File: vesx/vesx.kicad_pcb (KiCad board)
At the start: 4 copper layers, 100 x 40 mm, 180 parts, among them J1 TYPE-C-31-M-12, J2 Conn_01x05, J3 Conn_01x06, J4 Conn_01x03, J5 Conn_01x04, J6 STLINK, J7 Conn_01x04, J8 CAN, U1 Opamp_Quad, U2 LM1117DT-3.3, U3 LM5164DDA, U4 TO220_replacement_module, U5 L6498DTR, U6 L6498DTR, U7 STM32F405RGTx, U8 L6498DTR, U9 SN65HVD230DR, Y2 8MHz

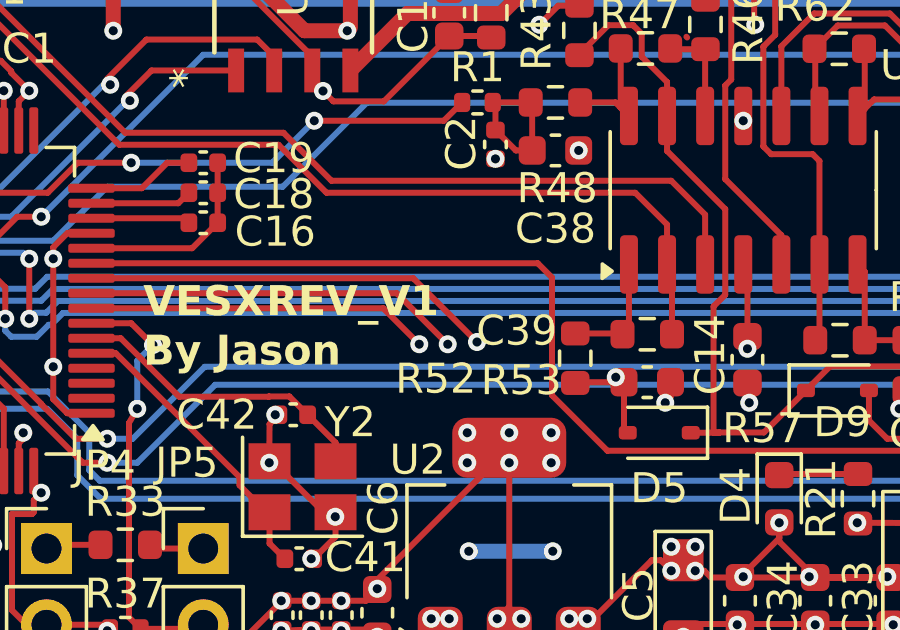
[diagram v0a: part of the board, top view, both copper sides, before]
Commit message: eeeeeeeeeeeeeeeeeeee
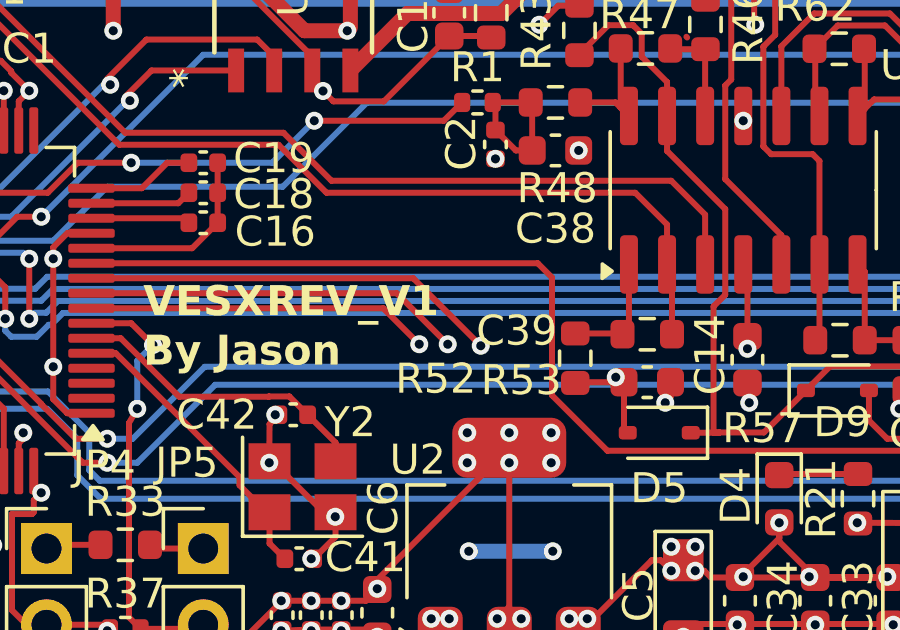
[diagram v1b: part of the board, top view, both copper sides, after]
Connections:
- C39 pad 1: CURRENT_A -> CURRENT_B
- C40 pad 1: CURRENT_B -> CURRENT_C
- D5 pad 2: CURRENT_A -> CURRENT_C
- R52 pad 2: CURRENT_A -> CURRENT_B
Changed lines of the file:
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@@
 			(layers "F.Cu" "F.Paste" "F.Mask")
 			(roundrect_rratio 0.25)
-			(net 48 "CURRENT_B")
+			(net 41 "CURRENT_C")
 			(pintype "passive")
 		)
@@
 			(layers "F.Cu" "F.Paste" "F.Mask")
 			(roundrect_rratio 0.25)
-			(net 34 "CURRENT_A")
+			(net 41 "CURRENT_C")
 			(pinfunction "A")
 			(pintype "passive")
@@
 			(layers "F.Cu" "F.Paste" "F.Mask")
 			(roundrect_rratio 0.25)
-			(net 34 "CURRENT_A")
+			(net 48 "CURRENT_B")
 			(pintype "passive")
 		)
@@
 			(layers "F.Cu" "F.Paste" "F.Mask")
 			(roundrect_rratio 0.25)
-			(net 34 "CURRENT_A")
+			(net 48 "CURRENT_B")
 			(pintype "passive")
 		)
@@
 	)
 	(segment
-		(start 197.925 41.775)
-		(end 195.8 39.65)
+		(start 195.8 39.65)
+		(end 185.075 39.65)
 		(width 0.2)
 		(layer "F.Cu")
@@
 	)
 	(segment
-		(start 213.2 36.34)
-		(end 212.8 36.74)
+		(start 198.05 41.9)
+		(end 195.8 39.65)
 		(width 0.2)
 		(layer "F.Cu")
@@
 	)
 	(segment
-		(start 195.8 39.65)
-		(end 185.075 39.65)
+		(start 213.2 36.34)
+		(end 212.8 36.74)
 		(width 0.2)
 		(layer "F.Cu")
@@
 	)
 	(via
-		(at 197.925 41.775)
+		(at 198.05 41.9)
 		(size 0.6)
 		(drill 0.3)
@@
 	)
 	(segment
-		(start 197.925 41.775)
-		(end 202.7 37)
+		(start 198.05 41.9)
+		(end 202.95 37)
 		(width 0.2)
 		(layer "In2.Cu")
@@
 	)
 	(segment
-		(start 202.7 37)
+		(start 202.95 37)
 		(end 212.5 37)
 		(width 0.2)
